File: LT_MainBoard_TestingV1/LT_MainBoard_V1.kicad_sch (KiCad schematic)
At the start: 20 parts, among them CN1 NUCLEO-L432KC, J1 Molar Nanofit Connectors, U1 ISO1050DUB, U2 MCP2515-I/SO, U3 XBP9B-DPST-001, U4 LM7809_TO220, U5 LM7805_TO220, U6 LM3480-3.3

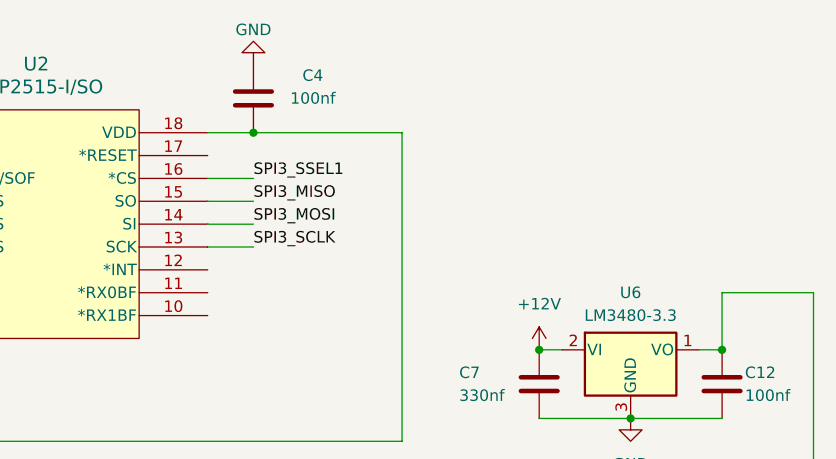
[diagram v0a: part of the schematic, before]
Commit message: Update Live Telemetry Board (11/19)
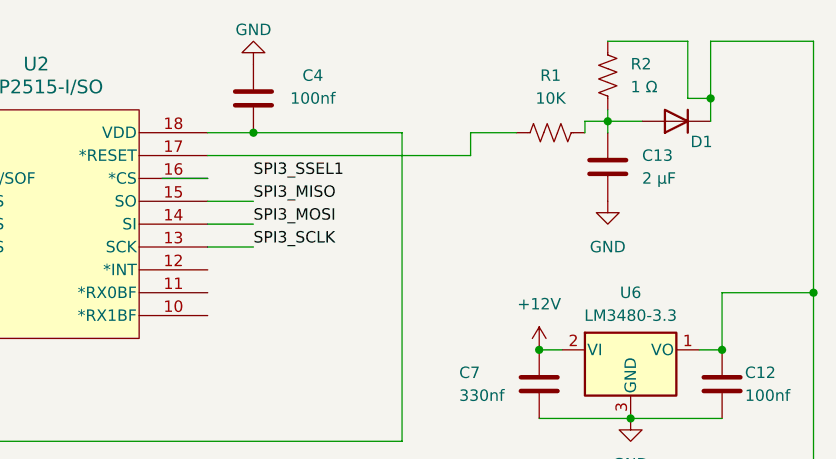
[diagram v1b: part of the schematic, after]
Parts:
- added C13: 2 µF, Capacitor_SMD:C_0805_2012Metric, symbol Device:C
- added D1: D, Diode_SMD:D_0805_2012Metric, symbol Device:D
- added R1: 10K, Resistor_SMD:R_0805_2012Metric, symbol Device:R_US
- added R2: 1 Ω, Resistor_SMD:R_0805_2012Metric, symbol Device:R_US
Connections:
- net GND: now also C13.2
- net SPI3_SSEL1: no longer U2.16 (*CS)
- net at C12.1, C3.2, C5.1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: now also D1.1 (K), R2.1
- net at U2.17 (*RESET): now also R1.1
- new net: C13.1, D1.2 (A), R1.2, R2.2

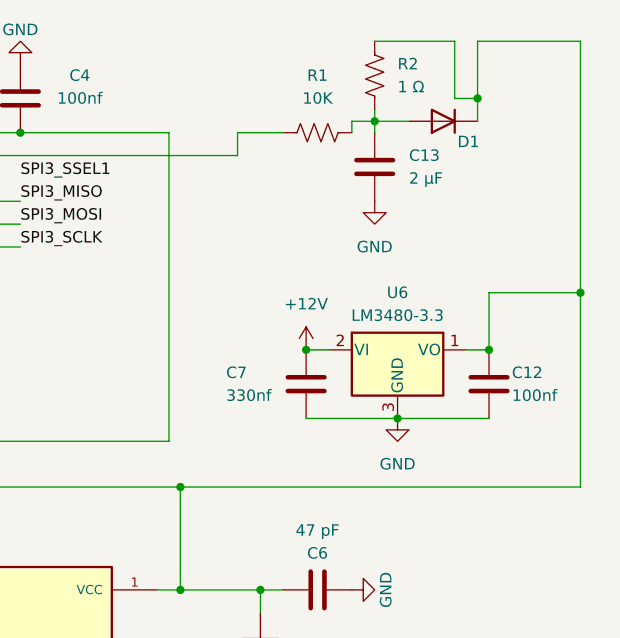
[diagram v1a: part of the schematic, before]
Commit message: Updated schematic (11/19)
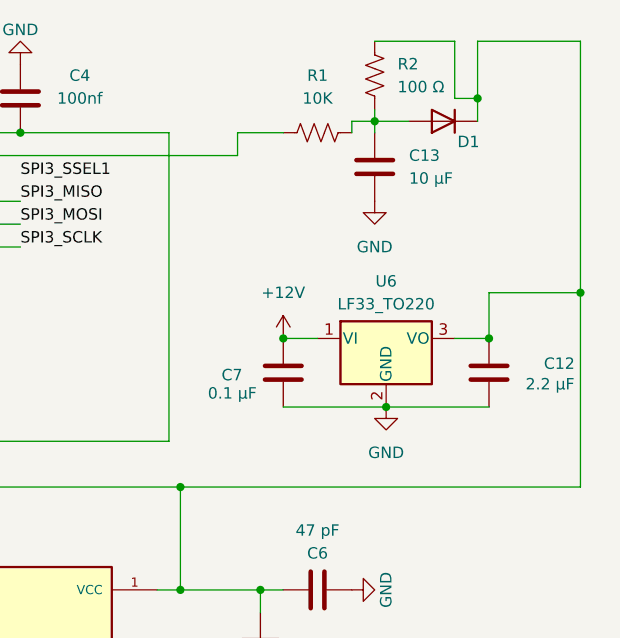
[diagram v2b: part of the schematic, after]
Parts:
- removed U6: LM3480-3.3, Package_TO_SOT_SMD:SOT-23, symbol Regulator_Linear:LM3480-3.3
- added U6: LF33_TO220, Package_TO_SOT_THT:TO-220-3_Vertical, symbol Regulator_Linear:LF33_TO220
- C12: value 100nf -> 2.2 µF; footprint Capacitor_SMD:C_0805_2012Metric_Pad1.18x1.45mm_HandSolder -> Capacitor_SMD:C_0805_2012Metric
- C13: value 2 µF -> 10 µF
- C7: value 330nf -> 0.1 µF; footprint Capacitor_SMD:C_0805_2012Metric_Pad1.18x1.45mm_HandSolder -> Capacitor_SMD:C_0805_2012Metric
- R2: value 1 Ω -> 100 Ω
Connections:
- net +12V: now also U6.1 (VI)
- net GND: now also U6.2 (GND)
- net at C12.1, C3.2, C5.1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: now also U6.3 (VO)
